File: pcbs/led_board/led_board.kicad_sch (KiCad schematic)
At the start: 4 parts, among them J1 JST S2B-ZR, U1 BCR401UW6Q-7

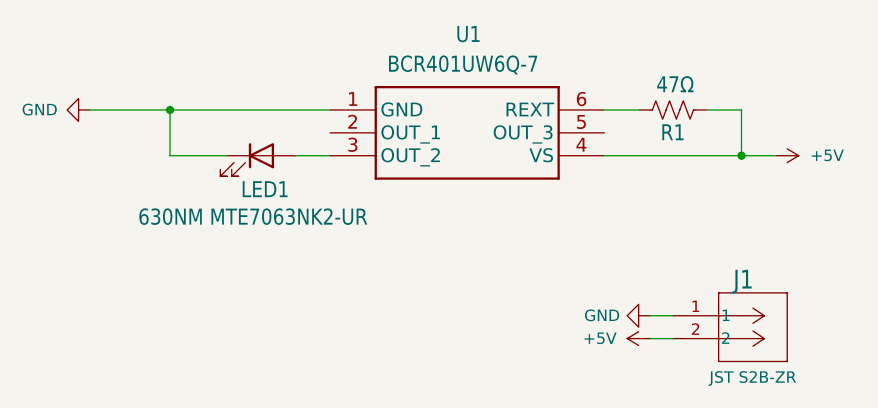
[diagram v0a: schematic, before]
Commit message: update led board to version 0.41
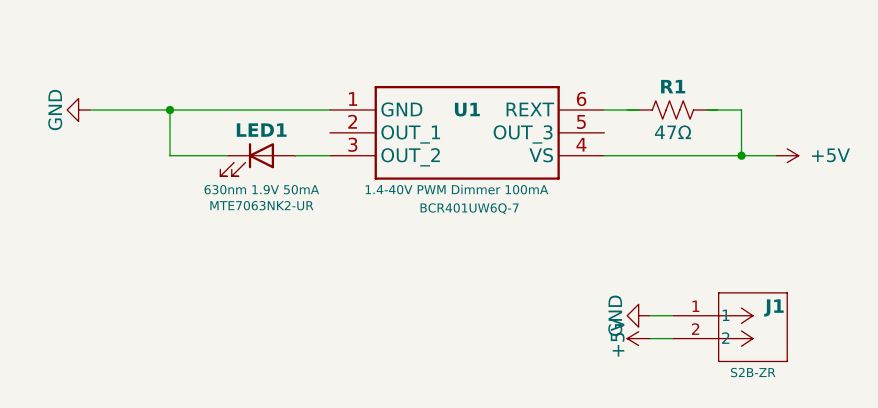
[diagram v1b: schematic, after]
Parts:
- J1: value JST S2B-ZR -> CONN HEADER R/A 2POS 1.5MM; footprint footprints:JST_ZH_2POS_RA_S2B-ZR -> footprints:JST_ZH_2POS_RA; symbol symbols:JST ZH 2POS R/A (S2B-ZRLFSN) -> symbols:JST ZH 2POS RA; DigiKeyURL (none) -> https://www.digikey.com/en/products/detail/jst-sales-americ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; MPN (none) -> S2B-ZR; URL https://www.digikey.com/en/products/detail/jst-sales-americ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 -> (none)
- LED1: value 630NM MTE7063NK2-UR -> 630nm 1.9V 50mA; symbol symbols:LED (MTE7063NK2-UR) -> symbols:LED_MTE7063NK2-UR; DigiKeyURL (none) -> https://www.digikey.com/en/products/detail/marktech-optoele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; MPN (none) -> MTE7063NK2-UR
- R1: footprint footprints:R_1206_3216Metric_Pad1.30x1.75mm_HandSolder -> footprints:R_1206
- U1: value BCR401UW6Q-7 -> 1.4-40V PWM Dimmer 100mA; footprint footprints:LED_driver_SOT-23-6_SOT95P285X140-6N -> footprints:SOT-23-6; symbol symbols:LED driver (BCR401UW6Q-7) -> symbols:LED_driver_BCR401UW6Q-7; DigiKeyURL (none) -> https://www.digikey.com/en/products/detail/diodes-incorpora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; MPN (none) -> BCR401UW6Q-7
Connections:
- net +5V: no longer R1.2
- net at R1.1: no longer U1.6 (REXT)
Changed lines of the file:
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@@
 		(dnp no)
 		(property "Reference" "R1"
+			(at 172.72 91.44 0)
+			(effects
+				(font
+					(size 1.5 1.5)
+					(thickness 0.3)
+					(bold yes)
+				)
+			)
+		)
+		(property "Value" "47Ω"
 			(at 172.72 96.52 0)
 			(effects
 				(font
-					(size 1.778 1.5113)
-				)
-			)
-		)
-		(property "Value" "47Ω"
-			(at 172.974 91.186 0)
-			(effects
-				(font
-					(size 1.778 1.5113)
-				)
-			)
-		)
-		(property "Footprint" "footprints:R_1206_3216Metric_Pad1.30x1.75mm_HandSolder"
+					(size 1.5 1.5)
+				)
+			)
+		)
+		(property "Footprint" "footprints:R_1206"
 			(at 171.704 93.726 90)
 			(effects
@@
 	)
 	(symbol
-		(lib_id "symbols:JST ZH 2POS R/A (S2B-ZRLFSN)")
+		(lib_id "symbols:JST ZH 2POS RA")
 		(at 172.72 116.84 0)
 		(unit 1)
@@
 		(dnp no)
 		(property "Reference" "J1"
-			(at 179.4246 114.0714 0)
-			(effects
-				(font
-					(size 2.083 1.7705)
-				)
-				(justify left bottom)
-			)
-		)
-		(property "Value" "JST S2B-ZR"
-			(at 181.61 123.698 0)
-			(effects
-				(font
-					(size 1.27 1.27)
-				)
-			)
-		)
-		(property "Footprint" "footprints:JST_ZH_2POS_RA_S2B-ZR"
+			(at 185.166 115.824 0)
+			(effects
+				(font
+					(size 1.5 1.5)
+					(thickness 0.3048)
+					(bold yes)
+				)
+				(justify right)
+			)
+		)
+		(property "Value" "CONN HEADER R/A 2POS 1.5MM"
+			(at 172.72 116.84 0)
+			(effects
+				(font
+					(size 1.524 1.524)
+				)
+				(hide yes)
+			)
+		)
+		(property "Footprint" "footprints:JST_ZH_2POS_RA"
 			(at 172.72 116.84 0)
 			(effects
@@
 			)
 		)
-		(property "URL" "https://www.digikey.com/en/products/detail/jst-sales-america-inc/S2B-ZR/926576"
+		(property "DigiKeyURL" "https://www.digikey.com/en/products/detail/jst-sales-america-inc/S2B-ZR/926576"
 			(at 172.72 116.84 0)
 			(effects
@@
 			)
 		)
+		(property "MPN" "S2B-ZR"
+			(at 181.61 123.19 0)
+			(effects
+				(font
+					(size 1 1)
+				)
+			)
+		)
 		(pin "1"
 		)
@@
 	)
 	(symbol
-		(lib_id "symbols:LED (MTE7063NK2-UR)")
+		(lib_id "symbols:LED_MTE7063NK2-UR")
 		(at 127 99.06 0)
 		(unit 1)
@@
 		(dnp no)
 		(property "Reference" "LED1"
-			(at 124.714 103.886 0)
-			(effects
-				(font
-					(size 1.778 1.5113)
-				)
-				(justify left bottom)
-			)
-		)
-		(property "Value" "630NM MTE7063NK2-UR"
-			(at 113.284 106.934 0)
-			(effects
-				(font
-					(size 1.778 1.5113)
-				)
-				(justify left bottom)
+			(at 127 96.266 0)
+			(effects
+				(font
+					(size 1.5 1.5)
+					(thickness 0.3)
+					(bold yes)
+				)
+			)
+		)
+		(property "Value" "630nm 1.9V 50mA"
+			(at 127 102.87 0)
+			(effects
+				(font
+					(size 1 1)
+				)
 			)
 		)
@@
 		)
 		(property "URL" "https://www.digikey.com/en/products/detail/marktech-optoelectronics/MTE7063NK2-UR/6817919"
+			(at 127 99.06 0)
+			(effects
+				(font
+					(size 1.27 1.27)
+				)
+				(hide yes)
+			)
+		)
+		(property "MPN" "MTE7063NK2-UR"
+			(at 127 104.648 0)
+			(effects
+				(font
+					(size 1 1)
+				)
+			)
+		)
+		(property "DigiKeyURL" "https://www.digikey.com/en/products/detail/marktech-optoelectronics/MTE7063NK2-UR/6817919"
 			(at 127 99.06 0)
 			(effects
@@
 		)
 		(property "Value" "GND"
-			(at 164.846 116.84 90)
-			(effects
-				(font
-					(size 1.27 1.27)
+			(at 166.37 116.84 0)
+			(effects
+				(font
+					(size 1.5 1.5)
 				)
 			)
@@
 		)
 		(property "Value" "+5V"
-			(at 164.592 119.38 90)
-			(effects
-				(font
-					(size 1.27 1.27)
+			(at 166.624 119.38 0)
+			(effects
+				(font
+					(size 1.5 1.5)
 				)
 			)
@@
 	)
 	(symbol
-		(lib_id "symbols:LED driver (BCR401UW6Q-7)")
+		(lib_id "symbols:LED_driver_BCR401UW6Q-7")
 		(at 134.62 93.98 0)
 		(unit 1)
@@
 		(dnp no)
 		(property "Reference" "U1"
-			(at 148.59 85.598 0)
-			(effects
-				(font
-					(size 1.778 1.5113)
+			(at 149.86 93.98 0)
+			(effects
+				(font
+					(size 1.5 1.5)
+					(thickness 0.3)
+					(bold yes)
+				)
+			)
+		)
+		(property "Value" "1.4-40V PWM Dimmer 100mA"
+			(at 138.43 102.87 0)
+			(effects
+				(font
+					(size 1 1)
 				)
 				(justify left)
 			)
 		)
-		(property "Value" "BCR401UW6Q-7"
-			(at 140.97 88.9 0)
-			(effects
-				(font
-					(size 1.778 1.5113)
-				)
-				(justify left)
-			)
-		)
-		(property "Footprint" "footprints:LED_driver_SOT-23-6_SOT95P285X140-6N"
+		(property "Footprint" "footprints:SOT-23-6"
 			(at 134.62 93.98 0)
 			(effects
@@
 			)
 		)
+		(property "MPN" "BCR401UW6Q-7"
+			(at 150.114 104.902 0)
+			(effects
+				(font
+					(size 1 1)
+				)
+			)
+		)
+		(property "DigiKeyURL" "https://www.digikey.com/en/products/detail/diodes-incorporated/BCR401UW6Q-7/7352843"
+			(at 134.62 93.98 0)
+			(effects
+				(font
+					(size 1.27 1.27)
+				)
+				(hide yes)
+			)
+		)
 		(pin "1"
 		)
@@
 		)
 		(property "Value" "GND"
-			(at 102.362 93.98 90)
-			(effects
-				(font
-					(size 1.27 1.27)
+			(at 104.14 93.98 0)
+			(effects
+				(font
+					(size 1.5 1.5)
 				)
 			)
@@
 		)
 		(property "Value" "+5V"
-			(at 187.96 99.0599 90)
-			(effects
-				(font
-					(size 1.27 1.27)
+			(at 187.96 99.06 90)
+			(effects
+				(font
+					(size 1.5 1.5)
 				)
 				(justify left)
